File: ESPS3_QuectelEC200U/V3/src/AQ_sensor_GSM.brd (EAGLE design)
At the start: 110 x 64 mm, 120 parts, among them IC1 MIC29302WU, J1 F-1X03-SIP-100-32, J3 PJ-002BH, Q1 MMBT2222, Q2 MMBT2222, Q3 MMBT2222, Q4 MMBT2222, Q5 MMBT2222, Q6 MMBT2222, Q7 MMBT2222, U3 TEXAS_INSTRUMENTS_LM1117IMP-3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, U5 TXS0108EPWR, X1 53048-08

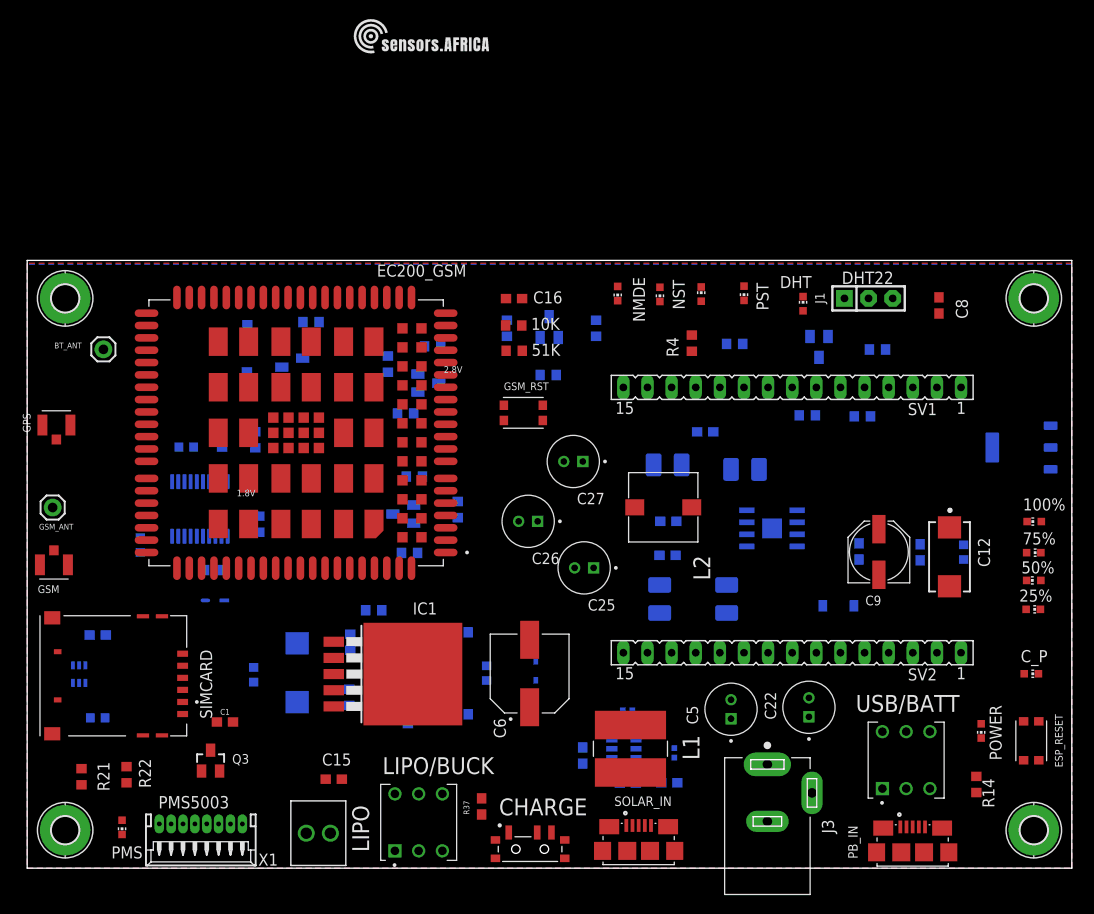
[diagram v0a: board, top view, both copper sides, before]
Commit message: V3 revised
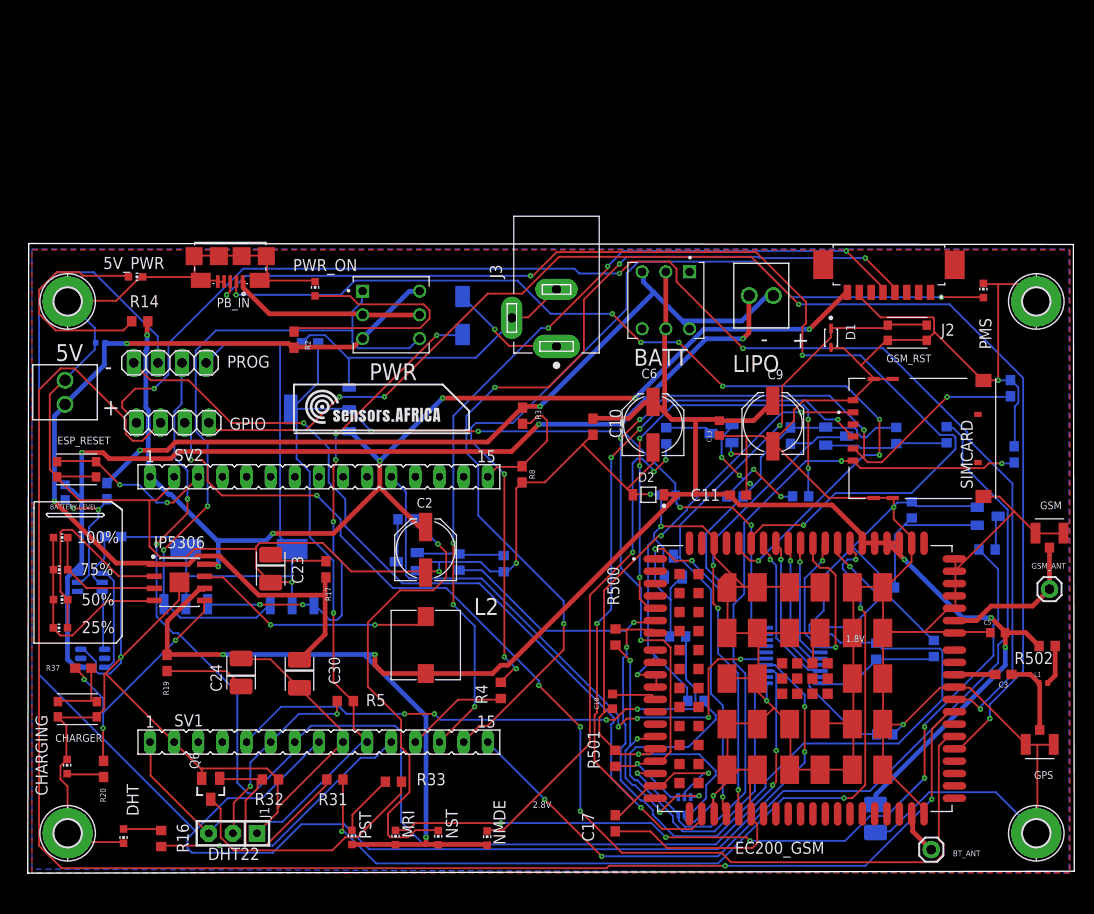
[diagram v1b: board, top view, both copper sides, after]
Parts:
- removed 10K, 51K: 4.7K, rcl:R0603
- removed C12: 470uf, T495X477K010ATE100:CAPMP7343X430N
- removed C14: 22nF, SparkFun-Capacitors:0402-TIGHT
- removed C22, C25, C26, C27: ECA-1HM220, Resistor_Capacitor:CAP_RADIAL_2MM
- removed C7: 100nf, 06035C104K4T2A:CAPC1608X90N
- removed CHARGE: PCM12SMTR, AQ_sensor_MRC:SW_PCM12SMTR
- removed C_P: ORANGE, led:CHIP-LED0603
- removed D5: ESD56151W04, 4.7V TVS Diode:DIO_1N4148WS_RR
- removed IC1: MIC29302WU, MIC29302WU:TO263-5
- removed LIPO/BUCK, USB/BATT: TL2285EE, TL2285EE:SW_TL2285EE
- removed POWER: RED, led:CHIP-LED0603
- removed Q1: MMBT2222, MMBT2222_:SOT23-BEC
- removed R1: 110k, SparkFun-Resistors:0603
- removed R11: 470R, rcl:R0603
- removed R6: 15, SparkFun-Resistors:0603
- removed R7: 10k, SparkFun-Resistors:0603
- removed SOLAR_IN: 10118192-0001LF, AQ_sensor_GSM:AMPHENOL_10118192-0001LF
- removed U$1: (no value), MT2492:SOT95P280X145-6N
- removed U$2: (no value), IP5306:SOIC127P600X165-9T209N
- removed X1: 53048-08, AQ_sensor_GSM:53048-08
- added 5V: 2828XX-2282834-2, Connector:TERMBLK_254-2N
- added 5V_PWR: RED, led:CHIP-LED0603
- added BATT, PWR: TL2285EE, TL2285EE:SW_TL2285EE
- added C4: 100nf, 06035C104K4T2A:CAPC1608X90N
- added CHARGER: KMR621NGLFS, AQ_sensor_GSM:SW_KMR621NGLFS
- added CHARGING, PWR_ON: ORANGE, led:CHIP-LED0603
- added D6: SS54-HF, SS54-HF schottkey Diode:DIOM5025X220N
- added DW01: DW01-P, DW01-P:SOT23-6L
- added GPIO, PROG: PINHD-1X4, Connector:1X04
- added IP5306: IP5306, IP5306:SOIC127P600X165-9T209N
- added J2: 53261-0871, 53261-0871:MOLEX_53261-0871
- added Q8: FS8205, FS8205:SOT95P280X145-6N
- added R500, R501: 4.7K, rcl:R0603
- added R502: 10R, rcl:R0603
- added VR1, VR2: LM7805MPX/NOPB, LM7805MPX_NOPB:VREG_LM7805MPX/NOPB
- C2: value 470uf -> 100uF; device T495X477K010ATE100:CAPMP7343X430N -> rcl:PANASONIC_D
- C3: value 100nf -> 100pF; device 06035C104K4T2A:CAPC1608X90N -> SparkFun-Capacitors:0603
- C5: value ECA-1HM220 -> 100nf; device Resistor_Capacitor:CAP_RADIAL_2MM -> 06035C104K4T2A:CAPC1608X90N
- C6: value EEEFN1C471P -> 100uF; device EEEFN1C471P:CAP_EEEFN1C471P -> rcl:PANASONIC_D
- L1: value 784787047 -> LQW15AN47NG00D; device Fixed Inductors:784787047 -> LQW15AN47NG00D 47uh:INDC1005X60N
- R10: value 47K -> 100R; device rcl:R0603 -> SparkFun-Resistors:0603
- R16, R4: value 470 -> 470R
- R2: value 51K -> 1k; device rcl:R0603 -> SparkFun-Resistors:0603
- R3: value 4.7K -> 47k; device rcl:R0603 -> SparkFun-Resistors:0603
- R8: value 47K -> 10k; device rcl:R0603 -> SparkFun-Resistors:0603
- R9: value 100k -> 1k; device rcl:R0603 -> SparkFun-Resistors:0603
- moved H3 116.7 mm to (106.3, 3.68), turned to 180 degrees
- moved H4 116.4 mm to (106.3, 59.7), turned to 180 degrees
- moved H2 116.3 mm to (4.26, 3.68), turned to 180 degrees
- moved H1 116.0 mm to (4.26, 59.7), turned to 180 degrees
- moved GPS 108.9 mm to (106.6, 13.0), turned to 180 degrees
- moved PMS 106.9 mm to (100.7, 60.8), turned to 0 degrees
- moved GSM_ANT 105.3 mm to (107.7, 29.4), turned to 180 degrees
- moved GSM 104.9 mm to (107.7, 35.3), turned to 0 degrees
- moved ESP_RESET 104.5 mm to (5.21, 42.0), turned to 180 degrees
- moved 100% 102.5 mm to (3.52, 34.8), turned to 270 degrees
- moved 50% 102.5 mm to (3.52, 28.3), turned to 270 degrees
- moved 75% 102.5 mm to (3.52, 31.4), turned to 90 degrees
- moved 25% 102.5 mm to (3.50, 25.3), turned to 90 degrees
- moved BT_ANT 101.9 mm to (95.2, 1.96), turned to 180 degrees
- moved R14 100.7 mm to (11.9, 57.6), turned to 0 degrees
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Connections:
- net USB_VBUS renamed G_USB_VBUS
- removed net +5V: R14.2, SV2.1, U3.3, USB/BATT.3, USB/BATT.4, X1.8
- removed net 3.8V: C6.1, C7.2, D5.C, IC1.4, LIPO/BUCK.1, LIPO/BUCK.6, R11.2, R9.2
- removed net 4.2V: C29.1, L2.2, LIPO/BUCK.2, LIPO/BUCK.5, R19.2, U$2.6
- removed net BVIN: C5.1, J3.1, R7.2, SOLAR_IN.1, U$1.5
- removed net D+: PB_IN.3, SOLAR_IN.3
- removed net D-: PB_IN.2, SOLAR_IN.2
- removed net N$11: R7.1, U$1.4
- removed net N$6: C14.2, L1.1, U$1.6
- removed net TF-CLK: SV2.7
- removed net TF-CS: SV2.9
- removed net TF-MISO: SV2.8
- removed net TF-MOSI: SV2.10
- removed net VUSB: C2.1, C3.2, IC1.2, PB_IN.1, R2.2, USB/BATT.1, USB/BATT.6
- new net 5VT: PB_IN.1, PWR.2, PWR.5
- new net BATT-: C4.2, DW01.6, LIPO.2, Q8.1
- new net BMSV: R3.2, R8.1, SV2.15
- new net G_ADC0: EC200_GSM.45, GPIO.1
- new net G_ADC1: EC200_GSM.44, GPIO.2
- new net G_ADC2: EC200_GSM.43
- new net G_GPIO1: EC200_GSM.126
- new net G_I2C_SCL: EC200_GSM.41, GPIO.4
- new net G_I2C_SDA: EC200_GSM.42, GPIO.3
- new net G_SPI_CLK: EC200_GSM.40
- new net G_SPI_CS: EC200_GSM.37
- new net G_SPI_MISO: EC200_GSM.39
- new net G_SPI_MOSI: EC200_GSM.38
- new net G_USB_BOOT: EC200_GSM.115, PROG.1
- new net G_USB_D+: EC200_GSM.69, PB_IN.3
- new net G_USB_D-: EC200_GSM.70, PB_IN.2
- new net LBV: BATT.3, BATT.4, LIPO.1, R10.2, R3.1
- new net N$19: DW01.3, Q8.4
- new net N$47: DW01.2, R9.1
- new net N$61: D6.2, J3.1
- new net N$9: DW01.1, Q8.6
- net 5V_IN: now also 5V.1, IP5306.1, PWR.3, PWR.4, R2.1; no longer C22.1, L1.2, R1.2, U$2.1
- net 5V_OUT: now also C2.+, IP5306.8, J2.8, R14.2, SV2.1, U3.3; no longer C25.1, C26.1, C27.1, U$2.8, USB/BATT.2, USB/BATT.5
- net GND: now also 5V.2, 5V_PWR.C, C2.-, C21.2, C5.1, C6.-, CHARGER.2_1, CHARGER.2_2, CHARGING.C, IP5306.9, J2.7, PROG.4, PWR_ON.C, Q8.3, R8.2, R9.2, VR1.2, VR1.4, VR2.2, VR2.4; no longer C12.2, C2.2, C22.2, C25.2, C26.2, C27.2, C3.1, C5.2, C6.2, C7.1, CHARGE.2, C_P.C, D5.A, IC1.3, LIPO.2, POWER.C, R10.1, R11.1, R6.1, R8.1, SOLAR_IN.4, SOLAR_IN.5, SOLAR_IN.SH1, SOLAR_IN.SH2, SOLAR_IN.SH3, SOLAR_IN.SH4, SOLAR_IN.SH5, SOLAR_IN.SH6, U$1.2, U$2.9, X1.7
- net GNSS_ANT: now also C3.2; no longer GPS.1
- net MCU_RXD: now also PROG.2
- net MCU_TXD: now also PROG.3
- net N$10: now also C3.1, GPS.1, L1.1; no longer C21.2, R1.1, R6.2, U$1.3
- net N$14: now also IP5306.4; no longer U$2.4
- net N$17: now also IP5306.2; no longer U$2.2
- net N$18: now also IP5306.3; no longer U$2.3
- net N$20: now also CHARGER.1_1, CHARGER.1_2; no longer CHARGE.1
- net N$21: now also IP5306.7; no longer U$2.7
- net N$25: now also 5V_PWR.A; no longer POWER.A
- net N$3: now also L1.2, R502.1; no longer C14.1, U$1.1
- net N$35: now also PWR_ON.A, R2.2; no longer IC1.1, Q1.C, R2.1
- net N$36: now also D6.1, VR1.1, VR2.1; no longer Q1.B, R3.2
- net N$37: now also C4.1, DW01.5, R10.1; no longer Q1.E, R8.2
- net N$38: now also PWR.1, PWR.6, VR1.3, VR2.3; no longer IC1.5, R10.2, R9.1
- net N$45: now also IP5306.5; no longer U$2.5
- net N$46: now also CHARGING.A; no longer C_P.A
- net PMS_RX: now also J2.5; no longer X1.5
- net PMS_TX: now also J2.4; no longer X1.4
- net SIMDATA: now also R501.1; no longer 10K.1
- net USIM_DET: now also R500.1; no longer 51K.1
- net USIM_VDD: now also R501.2; no longer 10K.2
- net VBAT_EN: no longer R3.1
- net VDD_EXT: now also R500.2; no longer 51K.2
- net V_LIPO: now also BATT.2, BATT.5, C29.1, C5.2, C6.+, IP5306.6, L2.2, R19.2, R502.2; no longer C12.1, LIPO.1, LIPO/BUCK.3, LIPO/BUCK.4
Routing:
- net GND: track 0.00 -> 870.1 mm, vias 0 -> 14
- net V_LIPO: track 0.00 -> 224.9 mm, vias 0 -> 6
- net MCU_RXD: track 0.00 -> 185.5 mm, vias 0 -> 2
- net G_ADC1: track 0.00 -> 175.1 mm, vias 0 -> 2
- net +3V3: track 0.00 -> 147.3 mm, vias 0 -> 5
- net G_ADC0: track 0.00 -> 144.2 mm, vias 0 -> 4
- net G_I2C_SCL: track 0.00 -> 141.3 mm, vias 0 -> 4
- net MCU_TXD: track 0.00 -> 137.2 mm, vias 0 -> 4
- net G_I2C_SDA: track 0.00 -> 122.5 mm, vias 0 -> 5
- net 5V_OUT: track 0.00 -> 120.6 mm, vias 0 -> 7
- net G_USB_D+: track 0.00 -> 119.3 mm, vias 0 -> 4
- net BATT-: track 0.00 -> 107.6 mm, vias 0 -> 3
- net SIMDATA: track 0.00 -> 100.9 mm, vias 0 -> 6
- net PMS_TX: track 0.00 -> 100.6 mm, vias 0 -> 4
- net G_USB_D-: track 0.00 -> 100.2 mm, vias 0 -> 8
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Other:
- board size 110 x 64 mm -> 110.2 x 66.3 mm
- board text added: "+"
- board text added: "-"
- board text added: "BATTERY LEVEL"
- board text removed: "PMS5003"
